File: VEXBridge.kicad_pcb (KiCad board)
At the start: 2 copper layers, 30 x 40 mm, 37 parts, among them J1 4P4C, J3 Conn_01x05_Pin, U1 LM2596S-5, U2 MAX481E, U5 SN74LVC2G14DBV

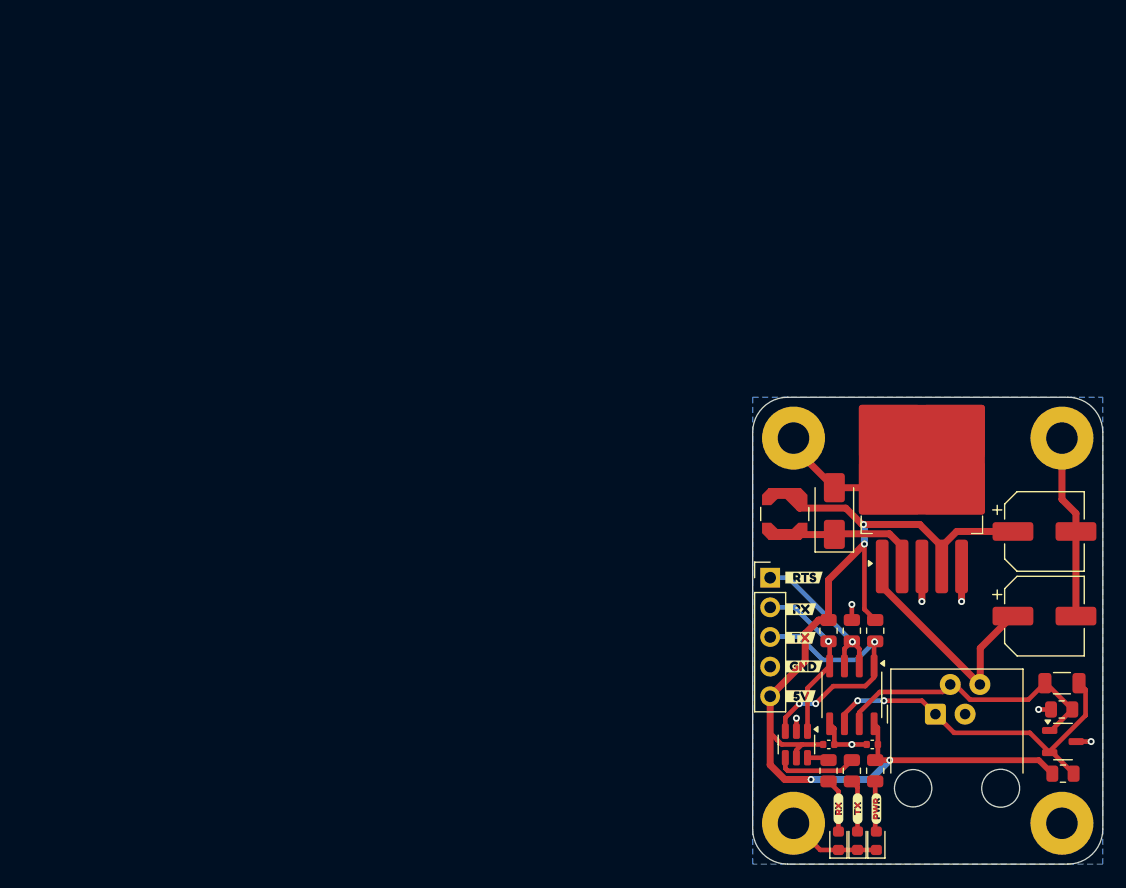
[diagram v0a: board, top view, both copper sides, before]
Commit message: VEXBridge v2 (WIP)
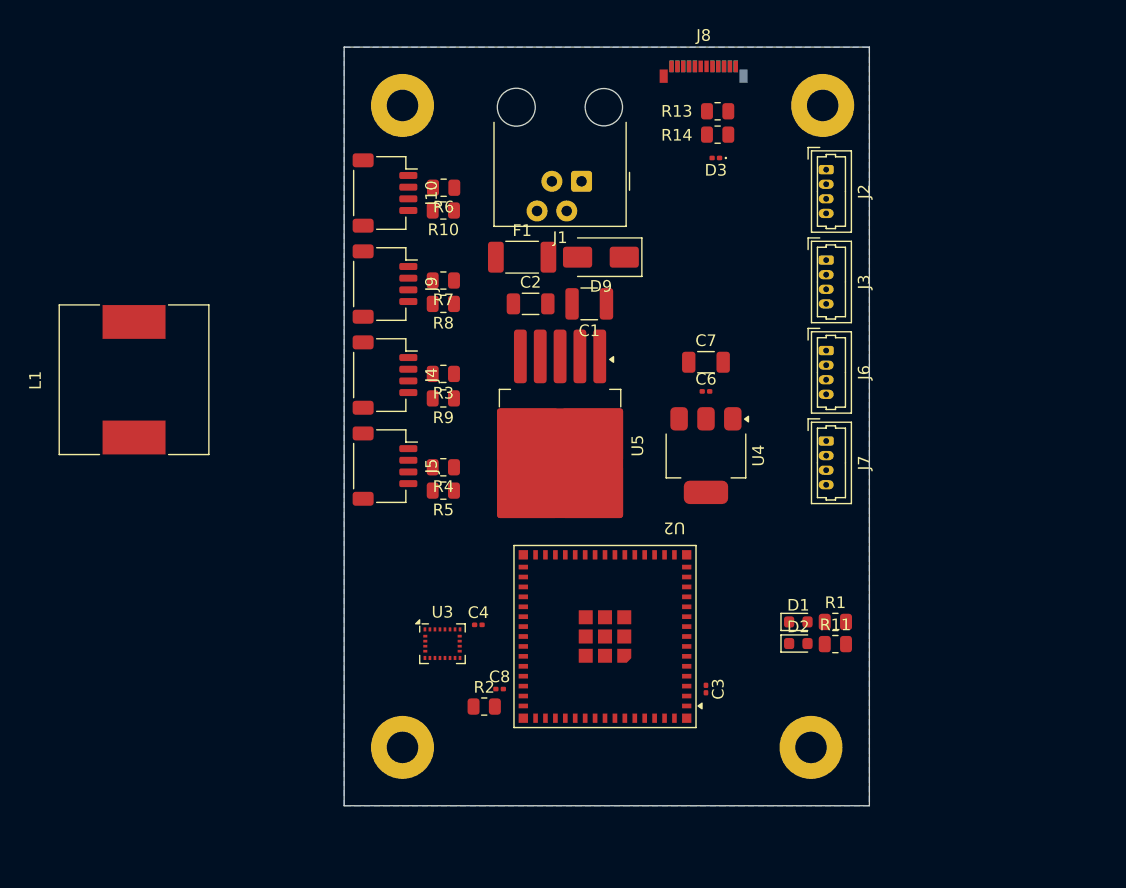
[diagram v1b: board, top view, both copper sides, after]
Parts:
- removed D4: ESDA5V3L, Package_TO_SOT_SMD:SOT-23-3
- removed U1: LM2596S-5, Package_TO_SOT_SMD:TO-263-5_TabPin3
- removed kibuzzard-675F6148: G***, kibuzzard-675F6148
- removed kibuzzard-675F61D9: G***, kibuzzard-675F61D9
- removed kibuzzard-675F61E2: G***, kibuzzard-675F61E2
- removed kibuzzard-675F61ED: G***, kibuzzard-675F61ED
- removed kibuzzard-675F6473: G***, kibuzzard-675F6473
- removed kibuzzard-675F648F: G***, kibuzzard-675F648F
- removed kibuzzard-675F6495: G***, kibuzzard-675F6495
- removed kibuzzard-676E54E7: G***, kibuzzard-676E54E7
- added C6: 10uF, Capacitor_SMD:C_0201_0603Metric, F.Cu at (81.0, 54.5)
- added C7: 22uF, Capacitor_SMD:C_1206_3216Metric, F.Cu at (81.0, 52.0)
- added C8: 1uF, Capacitor_SMD:C_0201_0603Metric, F.Cu at (63.3, 80.0)
- added F1: 1A, Fuse:Fuse_2010_5025Metric, F.Cu at (65.2, 43.0)
- added J10: QWIIC Connector, Connector_JST:JST_SH_SM04B-SRSS-TB_1x04-1MP_P1.00mm_Horizontal, F.Cu at (53.5, 37.5)
- added J2: Conn_01x04, Connector_Molex:Molex_PicoBlade_53047-0410_1x04_P1.25mm_Vertical, F.Cu at (91.3, 35.5)
- added J4: QWIIC Connector, Connector_JST:JST_SH_SM04B-SRSS-TB_1x04-1MP_P1.00mm_Horizontal, F.Cu at (53.5, 53.1)
- added J5: QWIIC Connector, Connector_JST:JST_SH_SM04B-SRSS-TB_1x04-1MP_P1.00mm_Horizontal, F.Cu at (53.5, 60.9)
- added J6: Conn_01x04, Connector_Molex:Molex_PicoBlade_53047-0410_1x04_P1.25mm_Vertical, F.Cu at (91.3, 51.0)
- added J7: Conn_01x04, Connector_Molex:Molex_PicoBlade_53047-0410_1x04_P1.25mm_Vertical, F.Cu at (91.3, 58.8)
- added J8: USB_C_Receptacle_USB2.0_14P, Connector_USB:USB_C_Plug_Molex_105444, F.Cu at (80.8, 26.6)
- added J9: QWIIC Connector, Connector_JST:JST_SH_SM04B-SRSS-TB_1x04-1MP_P1.00mm_Horizontal, F.Cu at (53.5, 45.3)
- added R10: 10k, Resistor_SMD:R_0805_2012Metric, F.Cu at (58.5, 39.0)
- added R11: 5.1k, Resistor_SMD:R_0805_2012Metric, F.Cu at (92.1, 76.2)
- added R13: 5.1k, Resistor_SMD:R_0805_2012Metric, F.Cu at (82.0, 30.5)
- added R14: 5.1k, Resistor_SMD:R_0805_2012Metric, F.Cu at (82.0, 32.5)
- added U3: LSM9DS1, Package_LGA:LGA-24L_3x3.5mm_P0.43mm, F.Cu at (58.4, 76.1)
- added U4: AMS1117-3.3, Package_TO_SOT_SMD:SOT-223-3_TabPin2, F.Cu at (81.0, 60.0)
- C1: value 100uF -> 220uF; footprint Capacitor_SMD:CP_Elec_6.3x7.7 -> Capacitor_SMD:C_1210_3225Metric
- C2: value 220uF -> 100uF; footprint Capacitor_SMD:CP_Elec_6.3x7.7 -> Capacitor_SMD:C_1206_3216Metric
- C3, C4: value 0.1uF -> 1uF; footprint Capacitor_SMD:C_0402_1005Metric -> Capacitor_SMD:C_0201_0603Metric
- D1: value LED -> RED
- D2: value LED -> GREEN
- D3: value LED -> D; footprint LED_SMD:LED_0603_1608Metric -> Diode_SMD:D_0201_0603Metric
- J3: value Conn_01x05_Pin -> Conn_01x04; footprint Connector_PinHeader_2.54mm:PinHeader_1x05_P2.54mm_Vertical -> Connector_Molex:Molex_PicoBlade_53047-0410_1x04_P1.25mm_Vertical
- L1: value 47uH -> 68uH; footprint Inductor_SMD:L_Coilcraft_LPS4018 -> Inductor_SMD:L_SXN_SMDRI127
- R1: value 100 -> 5.1k
- R2: value 120 -> 10k; footprint Resistor_SMD:R_1206_3216Metric -> Resistor_SMD:R_0805_2012Metric
- R3, R4: value 100 -> 10k
- U2: value MAX481E -> ESP32-S3-MINI-1U; footprint Package_SO:SOIC-8_3.9x4.9mm_P1.27mm -> RF_Module:ESP32-S2-MINI-1U
- U5: value SN74LVC2G14DBV -> LM2595S-5; footprint Package_TO_SOT_SMD:SOT-23-6 -> Package_TO_SOT_SMD:TO-263-5_TabPin3
- moved H1 83.5 mm to (55.0, 30.0)
- moved R6 73.0 mm to (58.5, 37.0), turned to 180 degrees
- moved H3 62.4 mm to (55.0, 85.0)
- moved D3 59.7 mm to (81.8, 34.5), turned to 180 degrees
- moved L1 56.9 mm to (32.0, 53.5)
- moved R5 56.2 mm to (58.5, 63.0)
- moved J1 54.8 mm to (70.3, 36.5), turned to 180 degrees
- moved R2 49.5 mm to (62.0, 81.5)
- moved C2 48.2 mm to (66.0, 47.0)
- moved R7 47.6 mm to (58.5, 45.0), turned to 180 degrees
- moved R3 47.4 mm to (58.5, 53.0), turned to 180 degrees
- moved C1 47.3 mm to (71.0, 47.0), turned to 180 degrees
- moved R8 44.8 mm to (58.5, 47.0), turned to 180 degrees
- moved R4 43.6 mm to (58.5, 61.0), turned to 180 degrees
- moved R9 38.5 mm to (58.5, 55.1), turned to 180 degrees
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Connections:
- C3 pad 1: +5V -> +3.3V
- C4 pad 1: +5V -> +3.3V
- D3 pad 1: GND -> +5V
- J1 pad 1: A -> unconnected-(J1-Pad1)
- J1 pad 2: B -> unconnected-(J1-Pad2)
- J1 pad 4: +12V -> Net-(F1-Pad1)
- J3 pad 1: RTS -> +5V
- J3 pad 2: RXD -> ENC_A1
- J3 pad 3: TXD -> ENC_B1
- R1 pad 1: +5V -> Net-(D1-A)
- R1 pad 2: Net-(D1-A) -> +3.3V
- R2 pad 1: B -> +3.3V
- R2 pad 2: A -> Net-(U2-EN)
- R3 pad 1: Net-(U5-1Y) -> +3.3V
- R3 pad 2: Net-(D2-A) -> SDA
- R4 pad 1: Net-(U5-2Y) -> +3.3V
- R4 pad 2: Net-(D3-A) -> SDA
- R5 pad 1: B -> +3.3V
- R5 pad 2: GND -> SCL
- R6 pad 1: +5V -> +3.3V
- R6 pad 2: A -> SDA
- R7 pad 1: +5V -> +3.3V
- R7 pad 2: TXD -> SDA
- R8 pad 1: RTS -> +3.3V
- R8 pad 2: GND -> SCL
- R9 pad 1: +5V -> +3.3V
- R9 pad 2: RXD -> SCL
- U2 pad 1: TXD -> GND
- U2 pad 2: RTS -> GND
- U2 pad 3: RTS -> +3.3V
- U2 pad 4: RXD -> SDA
- U2 pad 5: GND -> SCL
- U2 pad 6: A -> unconnected-(U2-IO2-Pad6)
- U2 pad 7: B -> unconnected-(U2-IO3-Pad7)
- U2 pad 8: +5V -> ENC_A1
- U5 pad 1: RXD -> Net-(D9-K)
- U5 pad 2: GND -> +12V
- U5 pad 3: TXD -> GND
- U5 pad 4: Net-(U5-2Y) -> +5V
- U5 pad 5: +5V -> GND
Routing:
- net +5V: track 91.8 -> 0.00 mm, vias 4 -> 0
- net GND: track 52.9 -> 0.00 mm, vias 7 -> 0
- net A: track 31.0 -> 0.00 mm, vias 2 -> 0
- net B: track 25.0 -> 0.00 mm
- net TXD: track 23.8 -> 0.00 mm, vias 3 -> 0
- net +12V: track 20.6 -> 0.00 mm
- net RXD: track 15.0 -> 0.00 mm, vias 1 -> 0
- net RTS: track 14.1 -> 0.00 mm, vias 1 -> 0
- net Net-(D9-K): track 12.2 -> 0.00 mm
- net Net-(U5-2Y): track 6.82 -> 0.00 mm
- net Net-(D2-A): track 4.65 -> 0.00 mm
- net Net-(D3-A): track 4.49 -> 0.00 mm
- net Net-(D1-A): track 4.34 -> 0.00 mm
- net Net-(U5-1Y): track 2.13 -> 0.00 mm
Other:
- board size 30 x 40 mm -> 45 x 65 mm

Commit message: Completed schematic
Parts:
- removed C1: 220uF, Capacitor_SMD:C_1210_3225Metric
- removed C2: 100uF, Capacitor_SMD:C_1206_3216Metric
- removed C3, C4, C8: 1uF, Capacitor_SMD:C_0201_0603Metric
- removed C6: 10uF, Capacitor_SMD:C_0201_0603Metric
- removed C7: 22uF, Capacitor_SMD:C_1206_3216Metric
- removed D1: RED, LED_SMD:LED_0603_1608Metric
- removed D2: GREEN, LED_SMD:LED_0603_1608Metric
- removed D3: D, Diode_SMD:D_0201_0603Metric
- removed D9: D_Schottky, Diode_SMD:D_SMA
- removed F1: 1A, Fuse:Fuse_2010_5025Metric
- removed G***: LOGO, LOGO
- removed H1, H2, H3, H4: MountingHole_Pad, MountingHole:MountingHole_2.7mm_M2.5_Pad
- removed J1: 4P4C, Connector_RJ:RJ9_Evercom_5301-440xxx_Horizontal
- removed J10, J4, J5, J9: QWIIC Connector, Connector_JST:JST_SH_SM04B-SRSS-TB_1x04-1MP_P1.00mm_Horizontal
- removed J2, J3, J6, J7: Conn_01x04, Connector_Molex:Molex_PicoBlade_53047-0410_1x04_P1.25mm_Vertical
- removed J8: USB_C_Receptacle_USB2.0_14P, Connector_USB:USB_C_Plug_Molex_105444
- removed L1: 68uH, Inductor_SMD:L_SXN_SMDRI127
- removed R1, R11, R13, R14: 5.1k, Resistor_SMD:R_0805_2012Metric
- removed R10, R2, R3, R4, R5, R6, R7, R8, R9: 10k, Resistor_SMD:R_0805_2012Metric
- removed U2: ESP32-S3-MINI-1U, RF_Module:ESP32-S2-MINI-1U
- removed U3: LSM9DS1, Package_LGA:LGA-24L_3x3.5mm_P0.43mm
- removed U4: AMS1117-3.3, Package_TO_SOT_SMD:SOT-223-3_TabPin2
- removed U5: LM2595S-5, Package_TO_SOT_SMD:TO-263-5_TabPin3
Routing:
- removed copper zone on B.Cu, net GND
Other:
- board outline removed
